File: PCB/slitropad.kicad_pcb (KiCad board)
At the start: 2 copper layers, 65.2 x 85.5 mm, 11 parts, among them SW1 SW_Push, SW2 SW_Push, SW3 SW_Push, SW4 SW_Push, SW5 SW_Push, SW6 SW_Push, SW7 SW_Push, SW8 SW_Push, SW9 SW_Push, U1 XIAO-RP2040-DIP

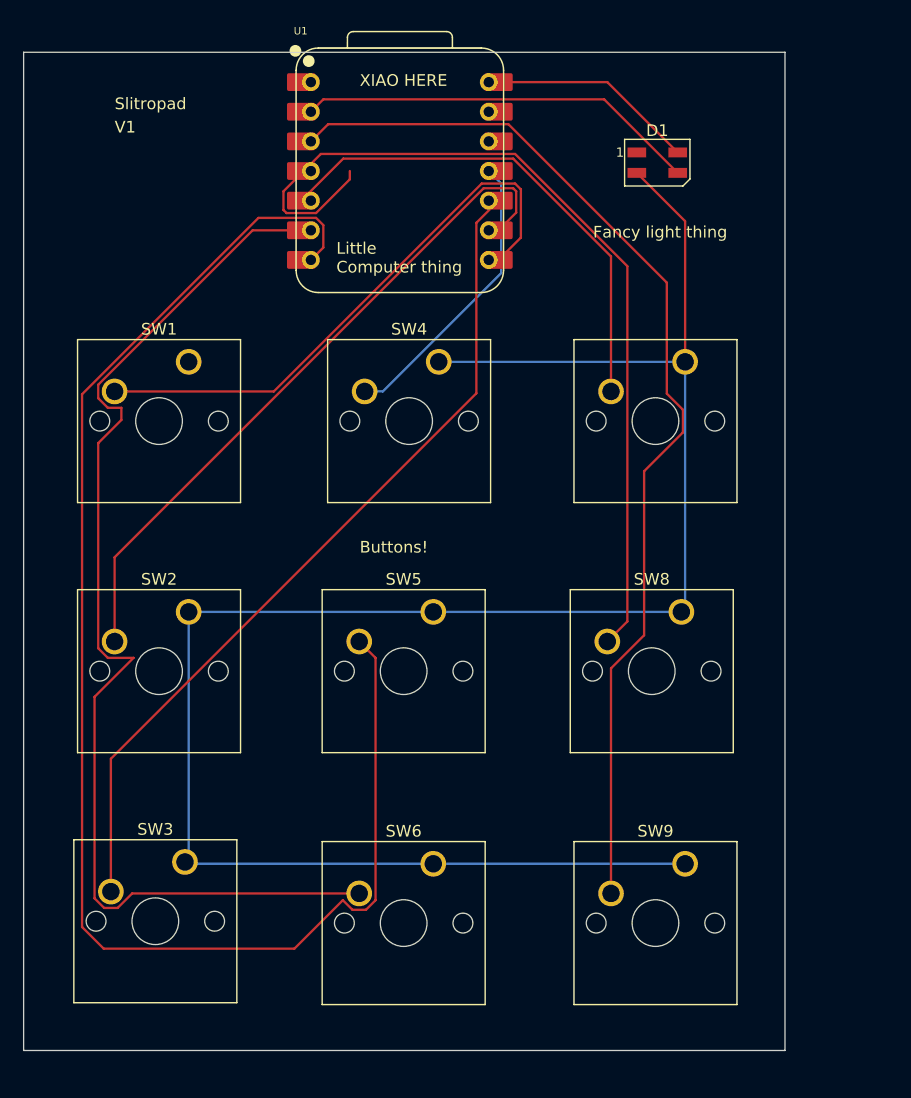
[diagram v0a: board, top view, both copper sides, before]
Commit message: push
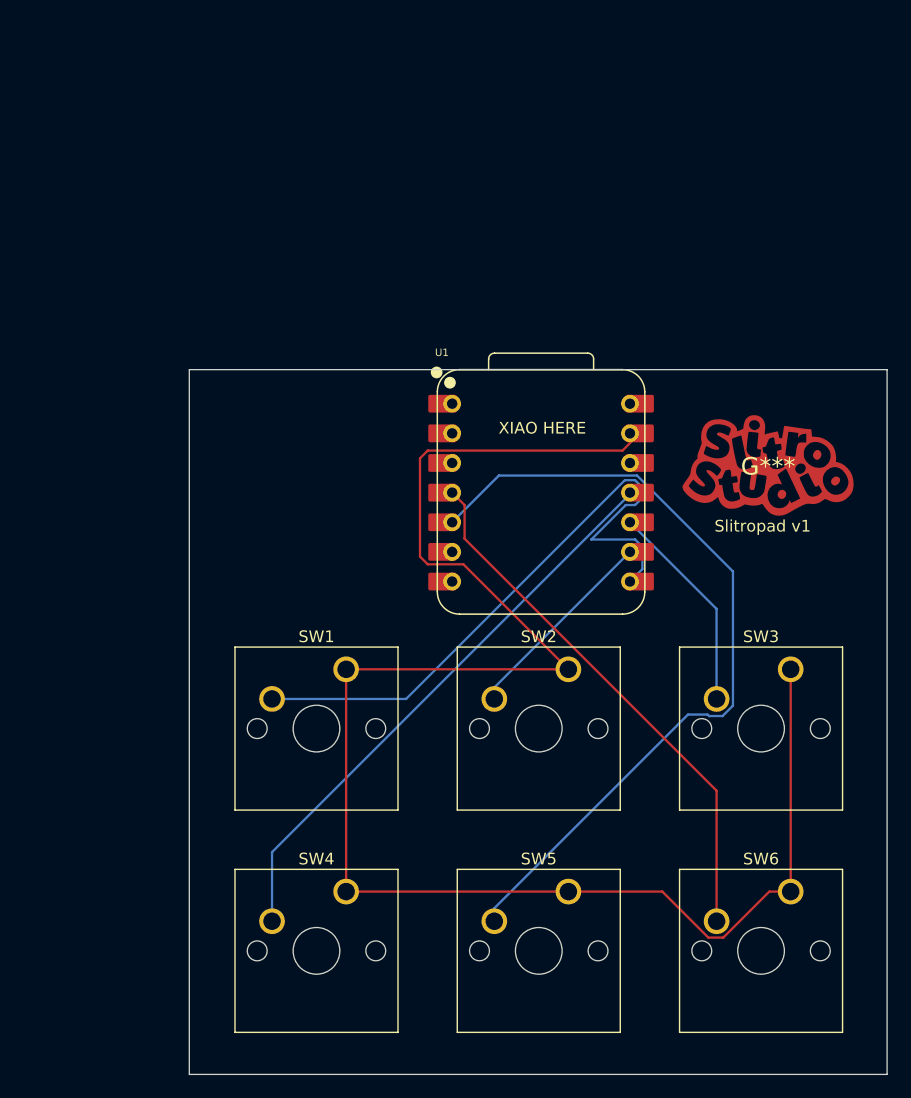
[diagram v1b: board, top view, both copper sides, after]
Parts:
- removed D1: SK6812MINI, LED_SMD:LED_SK6812MINI_PLCC4_3.5x3.5mm_P1.75mm
- removed SW7, SW8, SW9: SW_Push, Button_Switch_Keyboard:SW_Cherry_MX_1.00u_PCB
- added G***: LOGO, LOGO, F.Cu at (153.0, 58.5)
- U1: footprint footprint:XIAO-RP2040-DIP -> Xiao Foot:XIAO-RP2040-DIP
- moved SW3 54.5 mm to (154.9, 75.9)
- moved SW4 46.1 mm to (116.8, 94.9)
- moved SW2 32.9 mm to (135.9, 75.9)
- moved SW6 30.7 mm to (154.9, 94.9)
- moved U1 30.1 mm to (133.5, 60.7)
- moved SW1 29.6 mm to (116.8, 75.9)
- moved SW5 26.6 mm to (135.9, 94.9)
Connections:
- SW1 pad 1: GND -> Net-(U1-GND)
- SW2 pad 1: Net-(D1-VSS) -> Net-(U1-GND)
- SW3 pad 1: Net-(D1-VSS) -> Net-(U1-GND)
- SW4 pad 1: Net-(D1-VSS) -> Net-(U1-GND)
- SW5 pad 1: Net-(D1-VSS) -> Net-(U1-GND)
- SW5 pad 2: Net-(U1-GPIO0/TX) -> Net-(U1-GPIO6/SDA)
- SW6 pad 1: Net-(D1-VSS) -> Net-(U1-GND)
- SW6 pad 2: Net-(U1-GPIO7/SCL) -> Net-(U1-GPIO29/ADC3/A3)
- U1 pad 13: unconnected-(U1-GND-Pad13) -> Net-(U1-GND)
- U1 pad 14: Net-(D1-VDD) -> unconnected-(U1-VBUS-Pad14)
- U1 pad 2: Net-(D1-DIN) -> unconnected-(U1-GPIO27/ADC1/A1-Pad2)
- U1 pad 3: Net-(U1-GPIO28/ADC2/A2) -> unconnected-(U1-GPIO28/ADC2/A2-Pad3)
- U1 pad 6: Net-(U1-GPIO7/SCL) -> unconnected-(U1-GPIO7/SCL-Pad6)
- U1 pad 7: Net-(U1-GPIO0/TX) -> unconnected-(U1-GPIO0/TX-Pad7)
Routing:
- net Net-(D1-VSS): track 167.3 -> 0.00 mm
- net Net-(U1-GND): track 0.00 -> 143.4 mm
- net Net-(U1-GPIO0/TX): track 127.3 -> 0.00 mm
- net Net-(U1-GPIO7/SCL): track 97.5 -> 0.00 mm
- net Net-(U1-GPIO28/ADC2/A2): track 92.2 -> 0.00 mm
- net Net-(U1-GPIO4/MISO): track 73.0 -> 18.2 mm
- net Net-(U1-GPIO2/SCK): track 58.8 -> 17.4 mm
- net Net-(D1-DIN): track 34.5 -> 0.00 mm
- net Net-(U1-GPIO29/ADC3/A3): track 77.0 -> 46.1 mm
- net Net-(U1-GPIO6/SDA): track 43.1 -> 69.5 mm
- net Net-(U1-GPIO3/MOSI): track 25.1 -> 49.4 mm
- net Net-(D1-VDD): track 18.7 -> 0.00 mm
- net Net-(U1-GPIO1/RX): track 49.2 -> 54.6 mm
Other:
- board size 65.2 x 85.5 mm -> 59.8 x 60.4 mm
- board text added: "Slitropad v1"
- board text removed: "Buttons!"
- board text removed: "Fancy light thing"
- board text removed: "Little Computer thing"
- board text removed: "Slitropad"
- board text removed: "V1"
- board text removed: "Wrong way. Flip over."
